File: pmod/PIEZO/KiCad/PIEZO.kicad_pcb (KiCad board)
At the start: 2 copper layers, 37 x 32 mm, 8 parts, among them J1 Conn_01x06_Pin

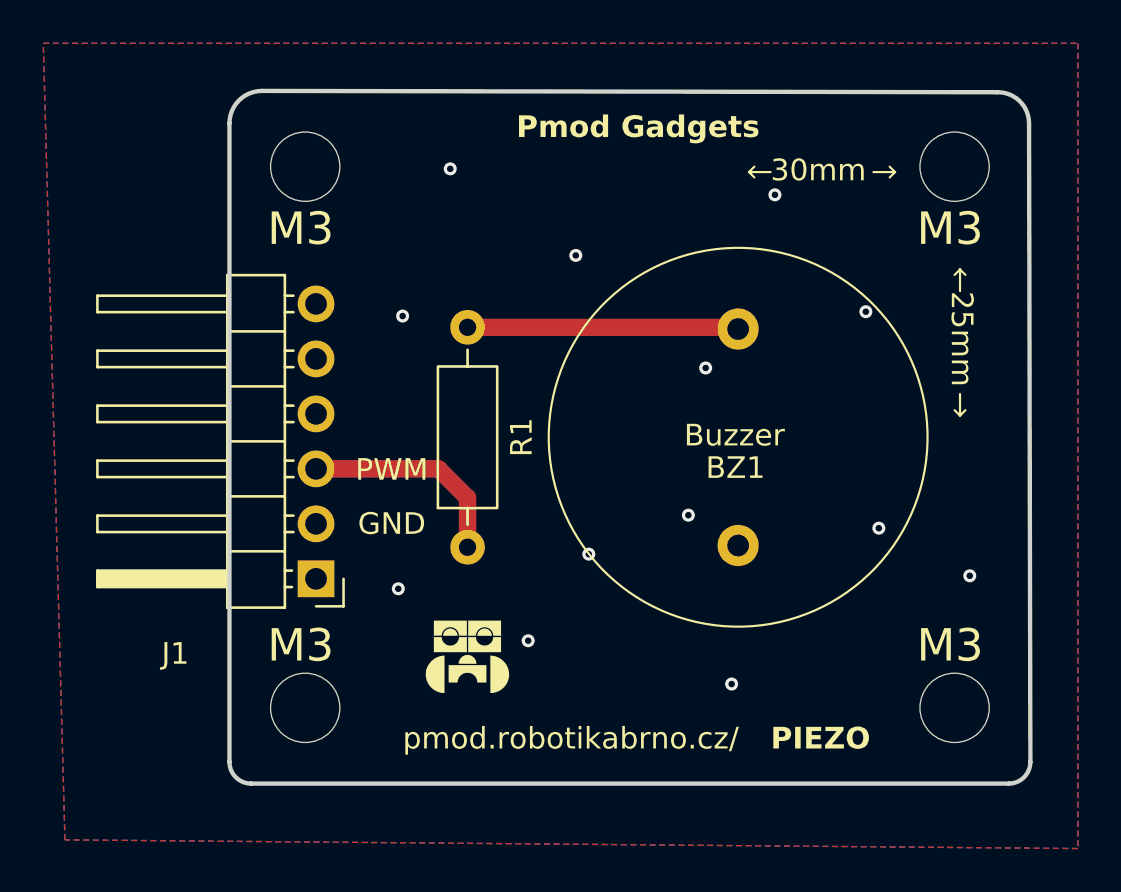
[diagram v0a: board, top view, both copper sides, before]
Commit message: jine piezo znovu
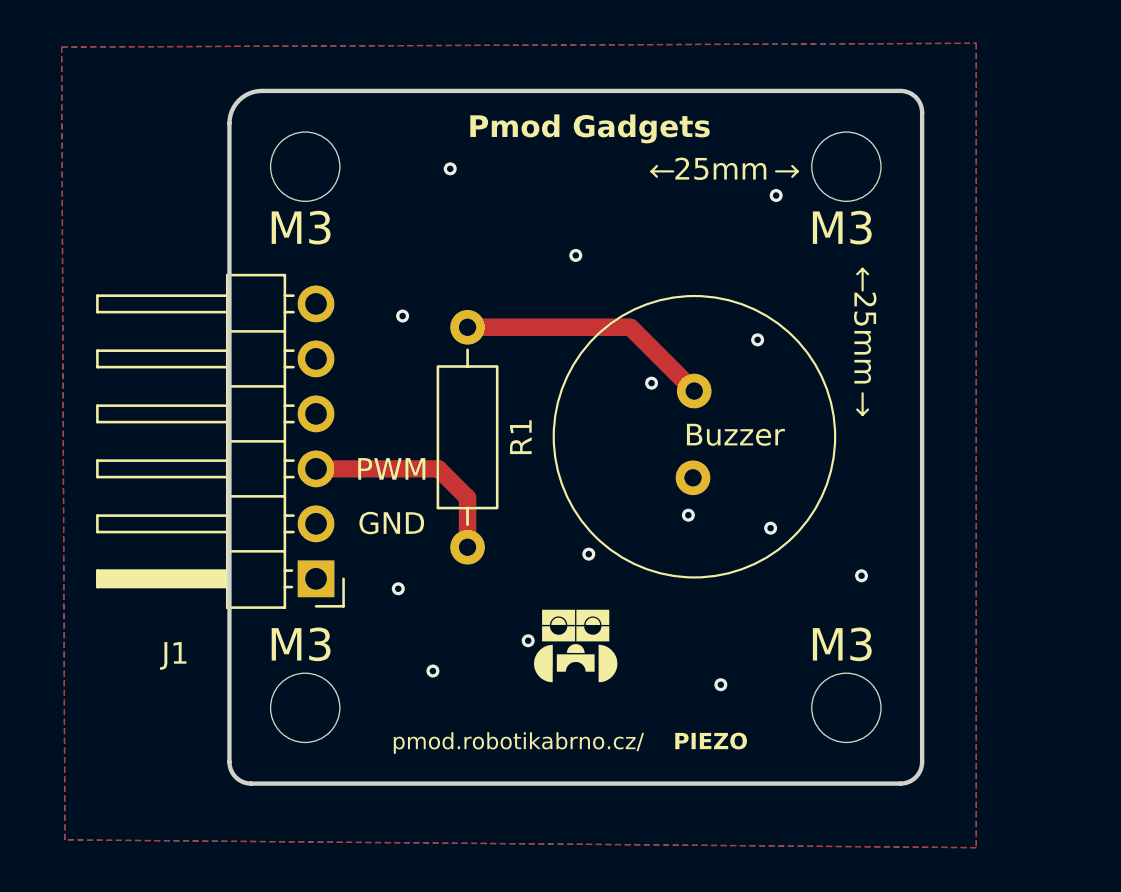
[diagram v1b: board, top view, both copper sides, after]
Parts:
- moved G*** 5.02 mm to (94.0, 72.5)
- moved REF** 5.00 mm to (106.5, 75.5)
- moved REF** 5.00 mm to (106.5, 50.5)
- moved BZ1 2.02 mm to (99.5, 63.0)
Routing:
- net Net-(BZ1-+): track 12.5 -> 11.7 mm
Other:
- board size 37 x 32 mm -> 32 x 32 mm
- board text removed: "30mm"
